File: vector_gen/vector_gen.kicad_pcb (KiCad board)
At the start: 2 copper layers, 98 parts, among them J1 ARDUINO POWER 3.3V, J10 ARDUINO J1, J11 Conn_01x08, J2 ARDUINO J3 3.3V, J3 ARDUINO J2 3.3V, J5 ARDUINO J1 3.3V, J6 Conn_01x03, J7 ARDUINO POWER, J8 ARDUINO J3, J9 ARDUINO J2, Q1 2N3904, U1 MCP4922, U10 MCP4922, U11 MCP4922, U12 4019, U13 LM336, U14 74HC86, U16 74LS07, U17 74LS07, U19 MAX4544, U5 4066, U6 MCP6292, U7 TL072IP, U8 TL072IP, U9 LM319

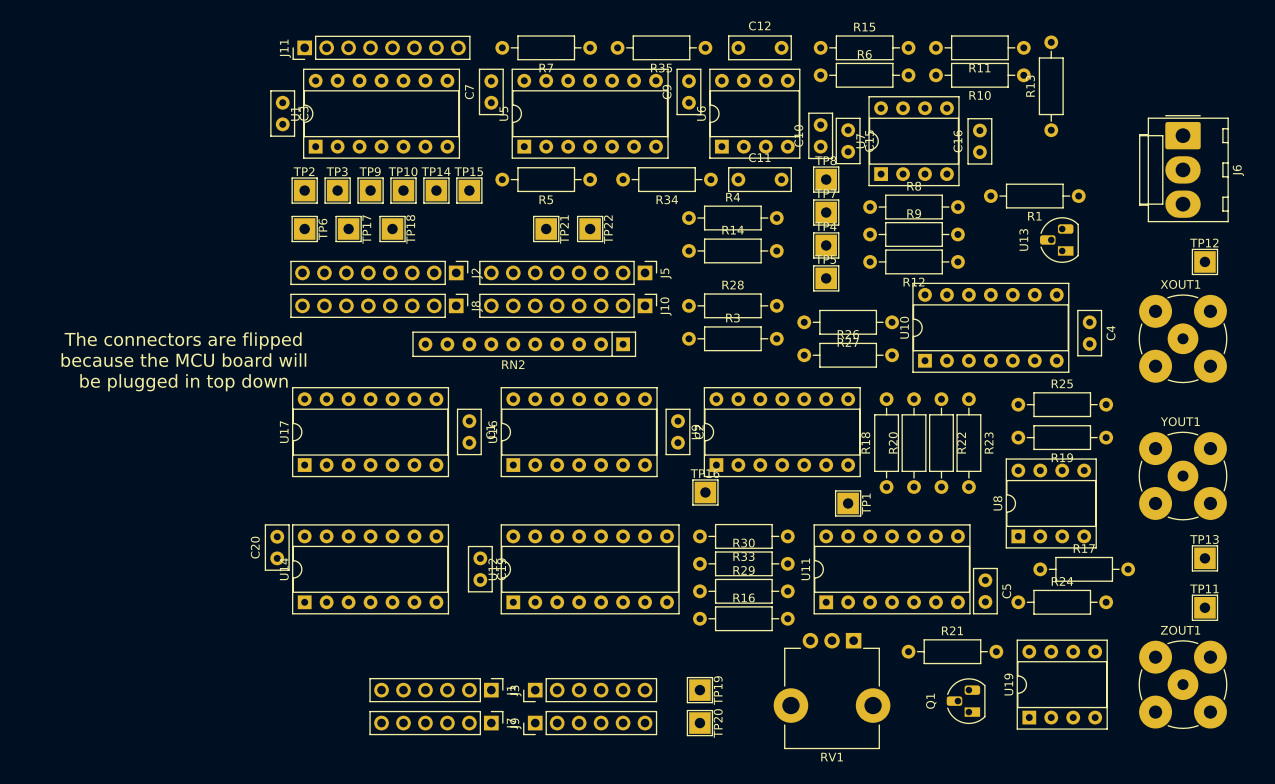
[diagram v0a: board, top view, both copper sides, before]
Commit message: PCB almost routed.
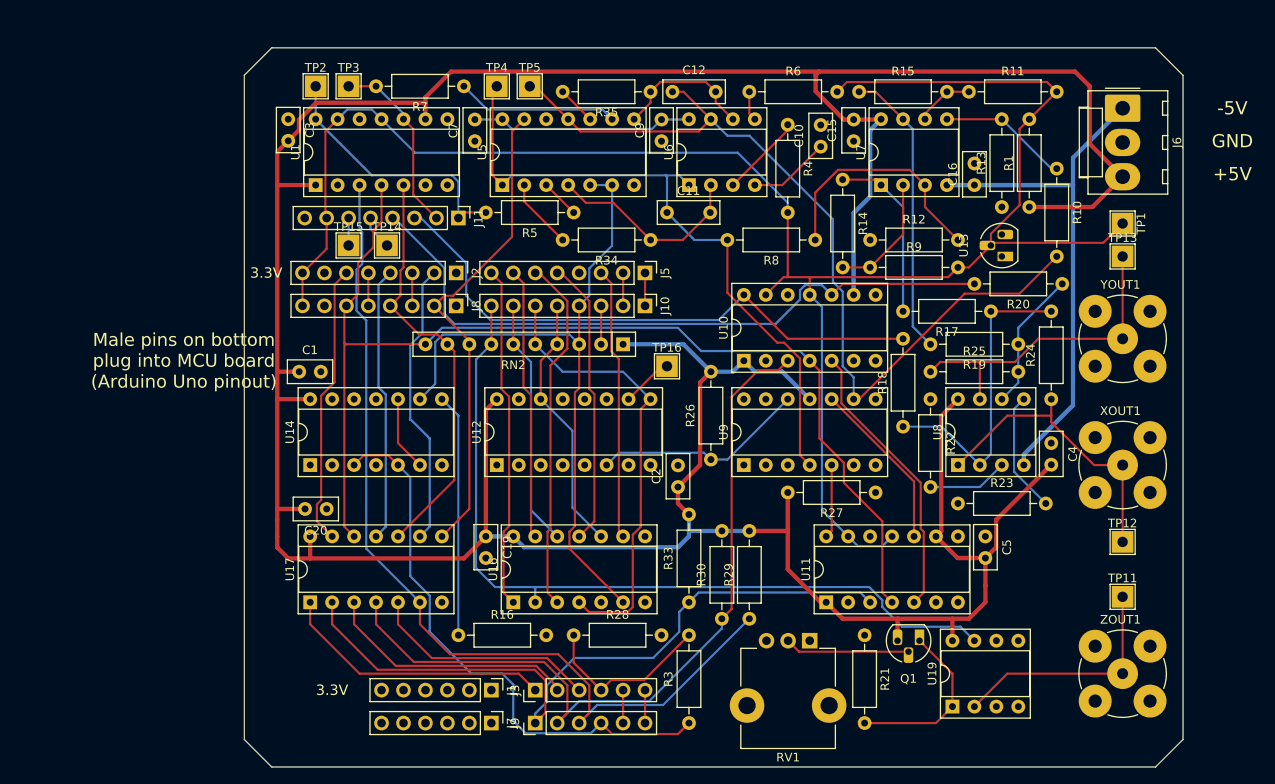
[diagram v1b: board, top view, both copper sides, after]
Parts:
- removed TP10, TP17, TP18, TP19, TP20, TP21, TP22, TP6, TP7, TP8, TP9: TestPoint, TestPoint:TestPoint_THTPad_2.5x2.5mm_Drill1.2mm
- moved TP1 45.4 mm to (42.5, -31.1)
- moved R3 44.5 mm to (-7.62, 26.7), turned to 90 degrees
- moved TP4 42.3 mm to (-29.8, -47.0)
- moved TP5 40.9 mm to (-26.0, -47.0)
- moved R28 40.4 mm to (-21.0, 16.5)
- moved TP13 36.2 mm to (42.5, -27.3)
- moved TP12 33.8 mm to (42.5, 5.71)
- moved R17 30.4 mm to (27.3, -21.0), turned to 180 degrees
- moved R20 29.1 mm to (35.6, -24.1), turned to 180 degrees
- moved R16 28.0 mm to (-34.3, 16.5)
- moved J11 26.5 mm to (-34.3, -31.8), turned to 270 degrees
- moved R24 23.8 mm to (34.3, -10.8), turned to 90 degrees
- moved U10 21.0 mm to (-1.27, -15.2)
- moved C1 20.5 mm to (-52.7, -14.0), turned to 0 degrees
- moved R27 19.8 mm to (14.0, 0.00)
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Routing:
- net +5V: track 0.00 -> 428.3 mm
- net Net-(J11-Pad7): track 0.00 -> 218.9 mm
- net Net-(J8-Pad6): track 0.00 -> 131.0 mm
- net Net-(J9-Pad3): track 0.00 -> 106.3 mm
- net Net-(C12-Pad1): track 0.00 -> 100.5 mm
- net Net-(J10-Pad8): track 0.00 -> 94.5 mm
- net Net-(J9-Pad2): track 0.00 -> 91.5 mm
- net Net-(J9-Pad1): track 0.00 -> 83.9 mm
- net Net-(J8-Pad4): track 0.00 -> 81.1 mm
- net Net-(J10-Pad4): track 0.00 -> 80.2 mm
- net Net-(J11-Pad4): track 0.00 -> 79.0 mm
- net Net-(C11-Pad1): track 0.00 -> 77.7 mm
- net Net-(J11-Pad3): track 0.00 -> 66.9 mm
- net Net-(J9-Pad4): track 0.00 -> 65.7 mm
- net -5V: track 0.00 -> 60.6 mm
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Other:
- board outline added: 108.6 x 83.2 mm
- board text added: "+5V"
- board text added: "-5V"
- board text added: "3.3V"
- board text added: "GND"
- board text added: "Male pins on bottom plug into MCU board (Arduino Uno pinout)"
- board text removed: "The connectors are flipped because the MCU board will be plugged in top down"
